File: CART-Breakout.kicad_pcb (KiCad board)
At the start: 2 copper layers, 47 x 50 mm, 11 parts, among them P1 Conn_01x05, P2 Conn_01x05, P3 Conn_01x05, P4 Conn_01x05, P5 Conn_01x05, P6 Conn_01x05

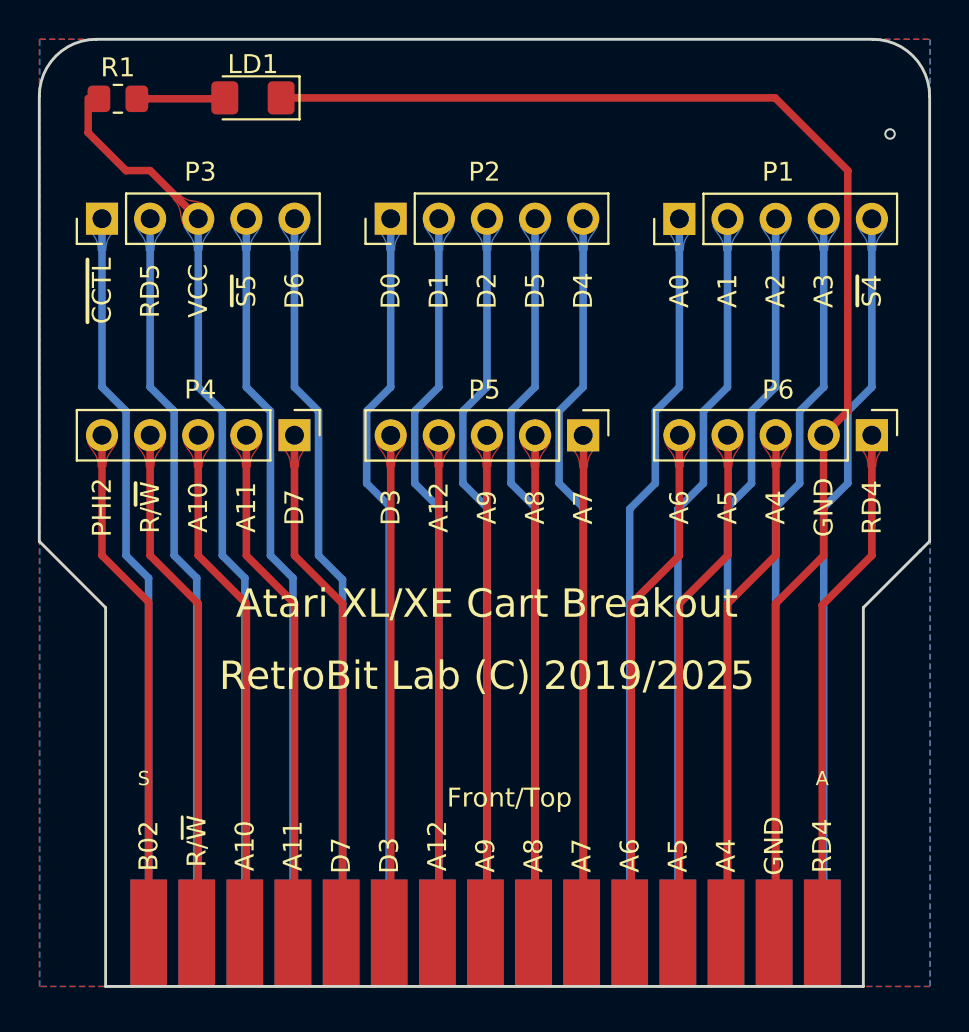
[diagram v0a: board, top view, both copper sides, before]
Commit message: Updated after KiCAD9 upgrade
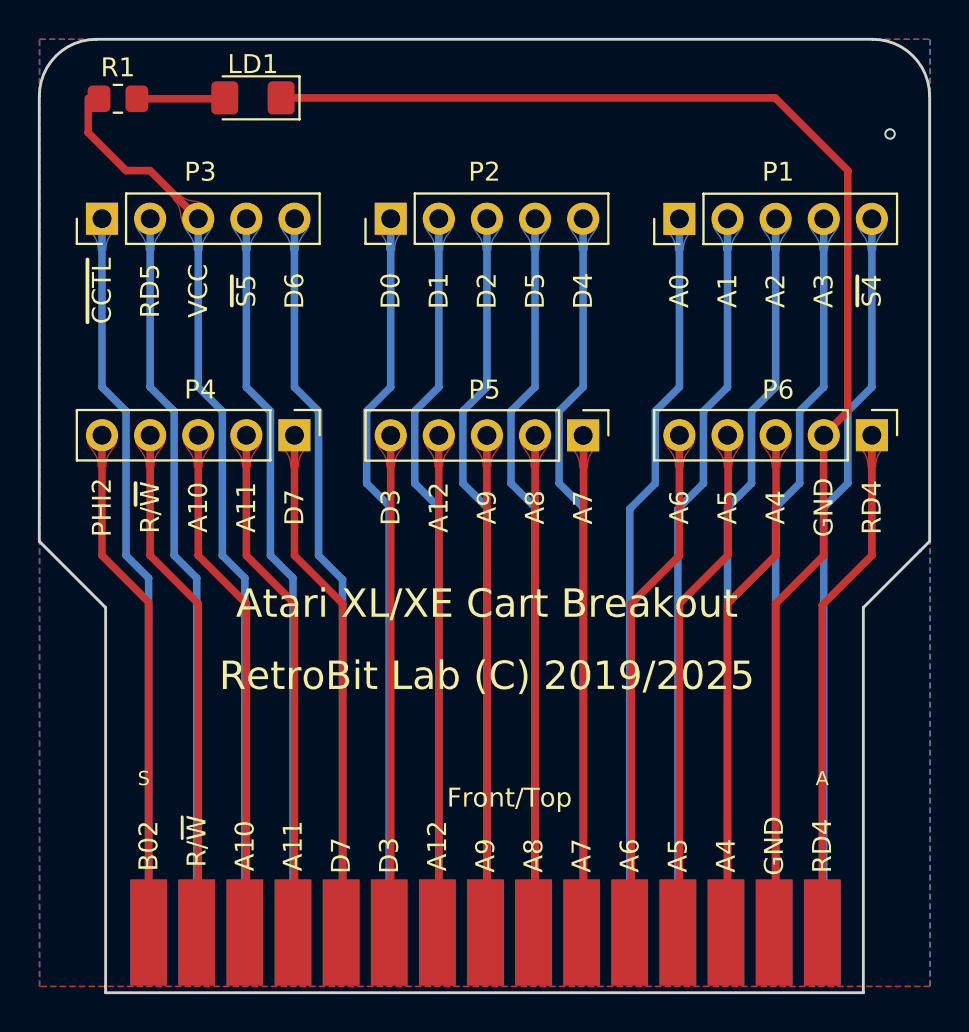
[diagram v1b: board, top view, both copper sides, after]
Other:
- board size 47 x 50 mm -> 47 x 50.3 mm
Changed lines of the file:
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@@
+	)
+	(gr_line
+		(start 131 118.33)
+		(end 131 118)
+		(stroke
+			(width 0.15)
+			(type default)
+		)
+		(layer "Edge.Cuts")
 	)
 	(gr_line
@@
 	)
 	(gr_line
-		(start 131 118)
-		(end 171 118)
-		(stroke
-			(width 0.15)
-			(type solid)
-		)
-		(layer "Edge.Cuts")
-	)
-	(gr_line
 		(start 174 95)
 		(end 174.5 94.5)
@@
 			(width 0.15)
 			(type solid)
+		)
+		(layer "Edge.Cuts")
+	)
+	(gr_line
+		(start 171 118.33)
+		(end 131 118.33)
+		(stroke
+			(width 0.15)
+			(type default)
 		)
 		(layer "Edge.Cuts")
@@
 	)
 	(gr_line
-		(start 171 118)
+		(start 171 118.33)
 		(end 171 98)
 		(stroke
@@
 		(layer "Margin")
 		(pts
-			(xy 174.5 118) (xy 127.5 118)
-		)
-		(height 54.5)
+			(xy 171 118) (xy 131 118)
+		)
+		(height -8.76)
+		(format
+			(prefix "")
+			(suffix "")
+			(units 3)
+			(units_format 0)
+			(precision 4)
+			(suppress_zeroes yes)
+		)
+		(style
+			(thickness 0.1)
+			(arrow_length 1.27)
+			(text_position_mode 0)
+			(arrow_direction outward)
+			(extension_height 0.58642)
+			(extension_offset 0.5)
+			(keep_text_aligned yes)
+		)
+		(gr_text "40"
+			(at 151 125.61 0)
+			(layer "Margin")
+			(effects
+				(font
+					(size 1 1)
+					(thickness 0.15)
+				)
+			)
+		)
+	)
+	(dimension
+		(type aligned)
+		(layer "Margin")
+		(pts
+			(xy 127.5 68) (xy 127.5 118)
+		)
+		(height 5.86)
+		(format
+			(prefix "")
+			(suffix "")
+			(units 3)
+			(units_format 0)
+			(precision 4)
+			(suppress_zeroes yes)
+		)
+		(style
+			(thickness 0.1)
+			(arrow_length 1.27)
+			(text_position_mode 0)
+			(arrow_direction outward)
+			(extension_height 0.58642)
+			(extension_offset 0.5)
+			(keep_text_aligned yes)
+		)
+		(gr_text "50"
+			(at 120.49 93 90)
+			(layer "Margin")
+			(effects
+				(font
+					(size 1 1)
+					(thickness 0.15)
+				)
+			)
+		)
+	)
+	(dimension
+		(type aligned)
+		(layer "Margin")
+		(pts
+			(xy 174.52674 68) (xy 127.5 68)
+		)
+		(height 8.915)
+		(format
+			(prefix "")
+			(suffix "")
+			(units 3)
+			(units_format 0)
+			(precision 4)
+			(suppress_zeroes yes)
+		)
+		(style
+			(thickness 0.1)
+			(arrow_length 1.27)
+			(text_position_mode 0)
+			(arrow_direction outward)
+			(extension_height 0.58642)
+			(extension_offset 0.5)
+			(keep_text_aligned yes)
+		)
+		(gr_text "47.0267"
+			(at 151.01337 57.935 0)
+			(layer "Margin")
+			(effects
+				(font
+					(size 1 1)
+					(thickness 0.15)
+				)
+			)
+		)
+	)
+	(dimension
+		(type aligned)
+		(layer "Margin")
+		(pts
+			(xy 171 118.33) (xy 171 98)
+		)
+		(height 6.85)
+		(format
+			(prefix "")
+			(suffix "")
+			(units 3)
+			(units_format 0)
+			(precision 4)
+			(suppress_zeroes yes)
+		)
+		(style
+			(thickness 0.1)
+			(arrow_length 1.27)
+			(text_position_mode 0)
+			(arrow_direction outward)
+			(extension_height 0.58642)
+			(extension_offset 0.5)
+			(keep_text_aligned yes)
+		)
+		(gr_text "20.33"
+			(at 176.7 108.165 90)
+			(layer "Margin")
+			(effects
+				(font
+					(size 1 1)
+					(thickness 0.15)
+				)
+			)
+		)
+	)
+	(dimension
+		(type aligned)
+		(layer "Margin")
+		(pts
+			(xy 171 118) (xy 131 118)
+		)
+		(height -6)
 		(format
 			(prefix "")
@@
 			(keep_text_aligned yes)
 		)
-		(gr_text "1.8504 in"
-			(at 151 61.7 0)
+		(gr_text "1.5748 in"
+			(at 151 122.2 0)
 			(layer "Margin")
 			(effects
@@
 		(layer "Margin")
 		(pts
-			(xy 171 118) (xy 131 118)
-		)
-		(height -8.76)
+			(xy 171 98) (xy 171 68)
+		)
+		(height 10.27)
 		(format
 			(prefix "")
@@
 			(keep_text_aligned yes)
 		)
-		(gr_text "40"
-			(at 151 125.61 0)
+		(gr_text "30"
+			(at 180.12 83 90)
 			(layer "Margin")
 			(effects
@@
 				)
 			)
-		)
-	)
-	(dimension
-		(type aligned)
-		(layer "Margin")
-		(pts
-			(xy 127.52674 68) (xy 127.5 118)
-		)
-		(height 22.565533)
-		(format
-			(prefix "")
-			(suffix "")
-			(units 3)
-			(units_format 0)
-			(precision 4)
-			(suppress_zeroes yes)
-		)
-		(style
-			(thickness 0.1)
-			(arrow_length 1.27)
-			(text_position_mode 0)
-			(arrow_direction outward)
-			(extension_height 0.58642)
-			(extension_offset 0.5)
-			(keep_text_aligned yes)
-		)
-		(gr_text "50"
-			(at 103.79784 92.987317 89.96935822)
-			(layer "Margin")
-			(effects
-				(font
-					(size 1 1)
-					(thickness 0.15)
-				)
-			)
-		)
-	)
-	(dimension
-		(type aligned)
-		(layer "Margin")
-		(pts
-			(xy 174.52674 68) (xy 127.5 68)
-		)
-		(height 8.915)
-		(format
-			(prefix "")
-			(suffix "")
-			(units 3)
-			(units_format 0)
-			(precision 4)
-			(suppress_zeroes yes)
-		)
-		(style
-			(thickness 0.1)
-			(arrow_length 1.27)
-			(text_position_mode 0)
-			(arrow_direction outward)
-			(extension_height 0.58642)
-			(extension_offset 0.5)
-			(keep_text_aligned yes)
-		)
-		(gr_text "47.0267"
-			(at 151.01337 57.935 0)
-			(layer "Margin")
-			(effects
-				(font
-					(size 1 1)
-					(thickness 0.15)
-				)
-			)
-		)
-	)
-	(dimension
-		(type aligned)
-		(layer "Margin")
-		(pts
-			(xy 171 118) (xy 171 98)
-		)
-		(height 10.78)
-		(format
-			(prefix "")
-			(suffix "")
-			(units 3)
-			(units_format 0)
-			(precision 4)
-			(suppress_zeroes yes)
-		)
-		(style
-			(thickness 0.1)
-			(arrow_length 1.27)
-			(text_position_mode 0)
-			(arrow_direction outward)
-			(extension_height 0.58642)
-			(extension_offset 0.5)
-			(keep_text_aligned yes)
-		)
-		(gr_text "20"
-			(at 180.63 108 90)
-			(layer "Margin")
-			(effects
-				(font
-					(size 1 1)
-					(thickness 0.15)
-				)
-			)
-		)
-	)
-	(dimension
-		(type aligned)
-		(layer "Margin")
-		(pts
-			(xy 171 98) (xy 171 118)
-		)
-		(height -8)
-		(format
-			(prefix "")
-			(suffix "")
-			(units 0)
-			(units_format 1)
-			(precision 4)
-		)
-		(style
-			(thickness 0.3)
-			(arrow_length 1.27)
-			(text_position_mode 0)
-			(arrow_direction outward)
-			(extension_height 0.58642)
-			(extension_offset 0)
-			(keep_text_aligned yes)
-		)
-		(gr_text "0.7874 in"
-			(at 177.2 108 90)
-			(layer "Margin")
-			(effects
-				(font
-					(size 1.5 1.5)
-					(thickness 0.3)
-				)
-			)
-		)
-	)
-	(dimension
-		(type aligned)
-		(layer "Margin")
-		(pts
-			(xy 131 68) (xy 131 118)
-		)
-		(height 20)
-		(format
-			(prefix "")
-			(suffix "")
-			(units 0)
-			(units_format 1)
-			(precision 4)
-		)
-		(style
-			(thickness 0.3)
-			(arrow_length 1.27)
-			(text_position_mode 0)
-			(arrow_direction outward)
-			(extension_height 0.58642)
-			(extension_offset 0)
-			(keep_text_aligned yes)
-		)
-		(gr_text "1.9685 in"
-			(at 109.2 93 90)
-			(layer "Margin")
-			(effects
-				(font
-					(size 1.5 1.5)
-					(thickness 0.3)
-				)
-			)
-		)
-	)
-	(dimension
-		(type aligned)
-		(layer "Margin")
-		(pts
-			(xy 171 118) (xy 131 118)
-		)
-		(height -6)
-		(format
-			(prefix "")
-			(suffix "")
-			(units 0)
-			(units_format 1)
-			(precision 4)
-		)
-		(style
-			(thickness 0.3)
-			(arrow_length 1.27)
-			(text_position_mode 0)
-			(arrow_direction outward)
-			(extension_height 0.58642)
-			(extension_offset 0)
-			(keep_text_aligned yes)
-		)
-		(gr_text "1.5748 in"
-			(at 151 122.2 0)
-			(layer "Margin")
-			(effects
-				(font
-					(size 1.5 1.5)
-					(thickness 0.3)
-				)
-			)
